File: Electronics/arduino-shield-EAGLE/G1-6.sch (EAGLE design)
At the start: 23 parts

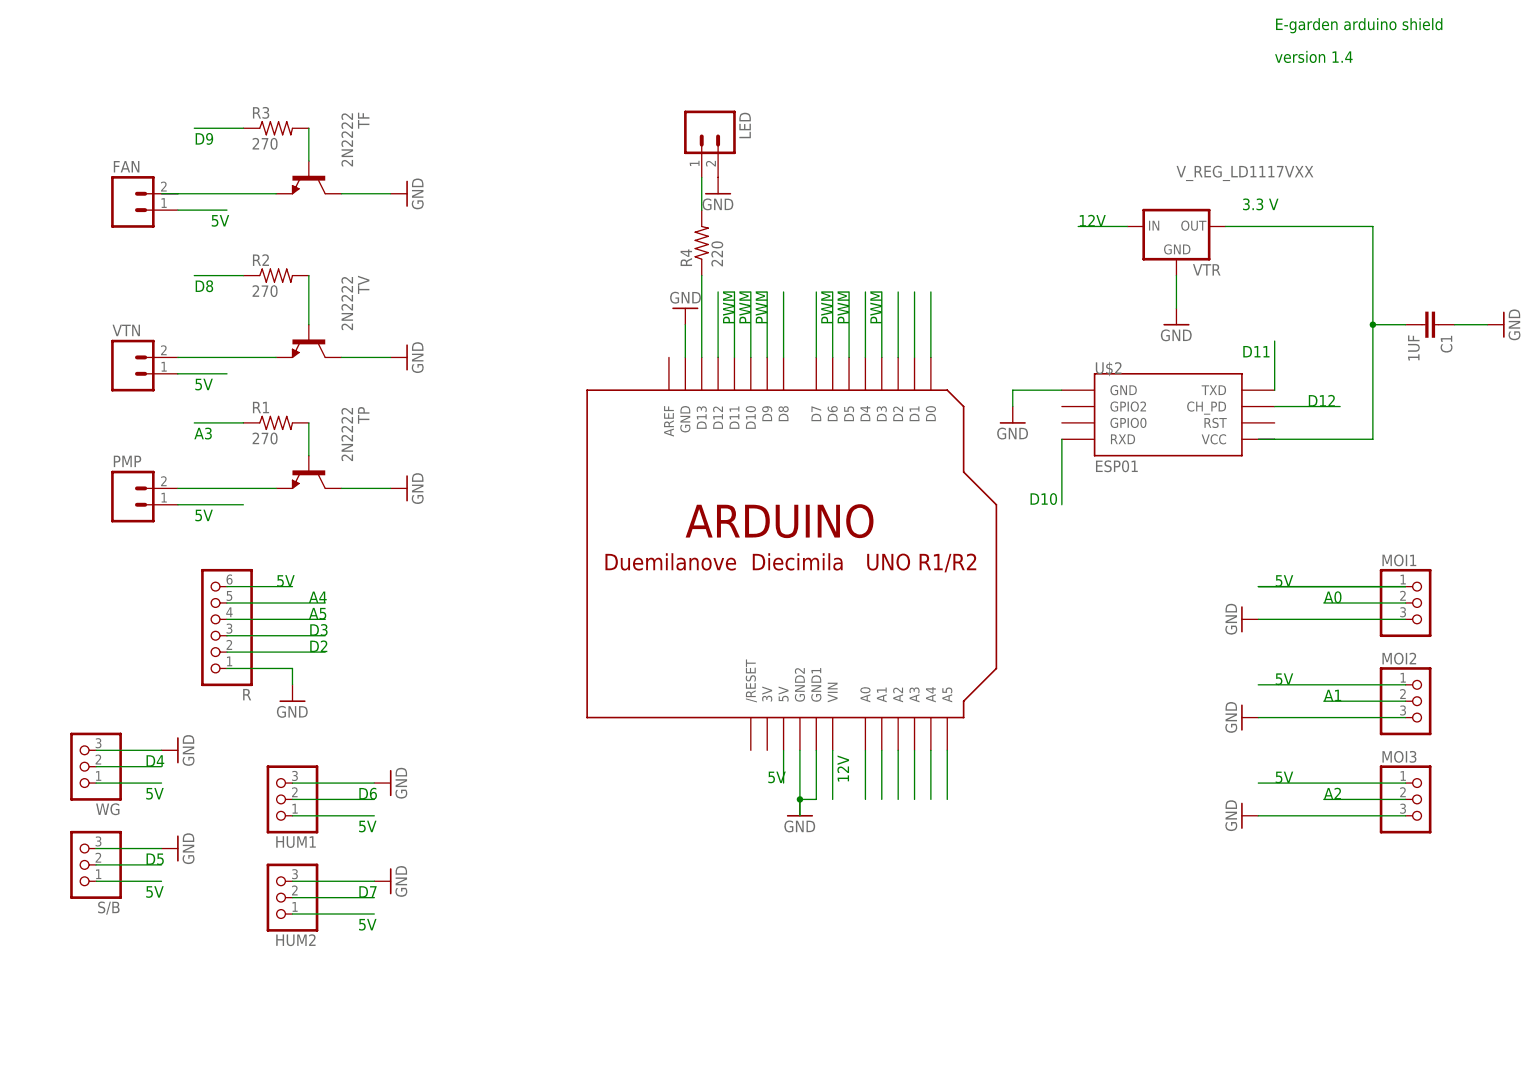
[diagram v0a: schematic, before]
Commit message: shield version 1.6
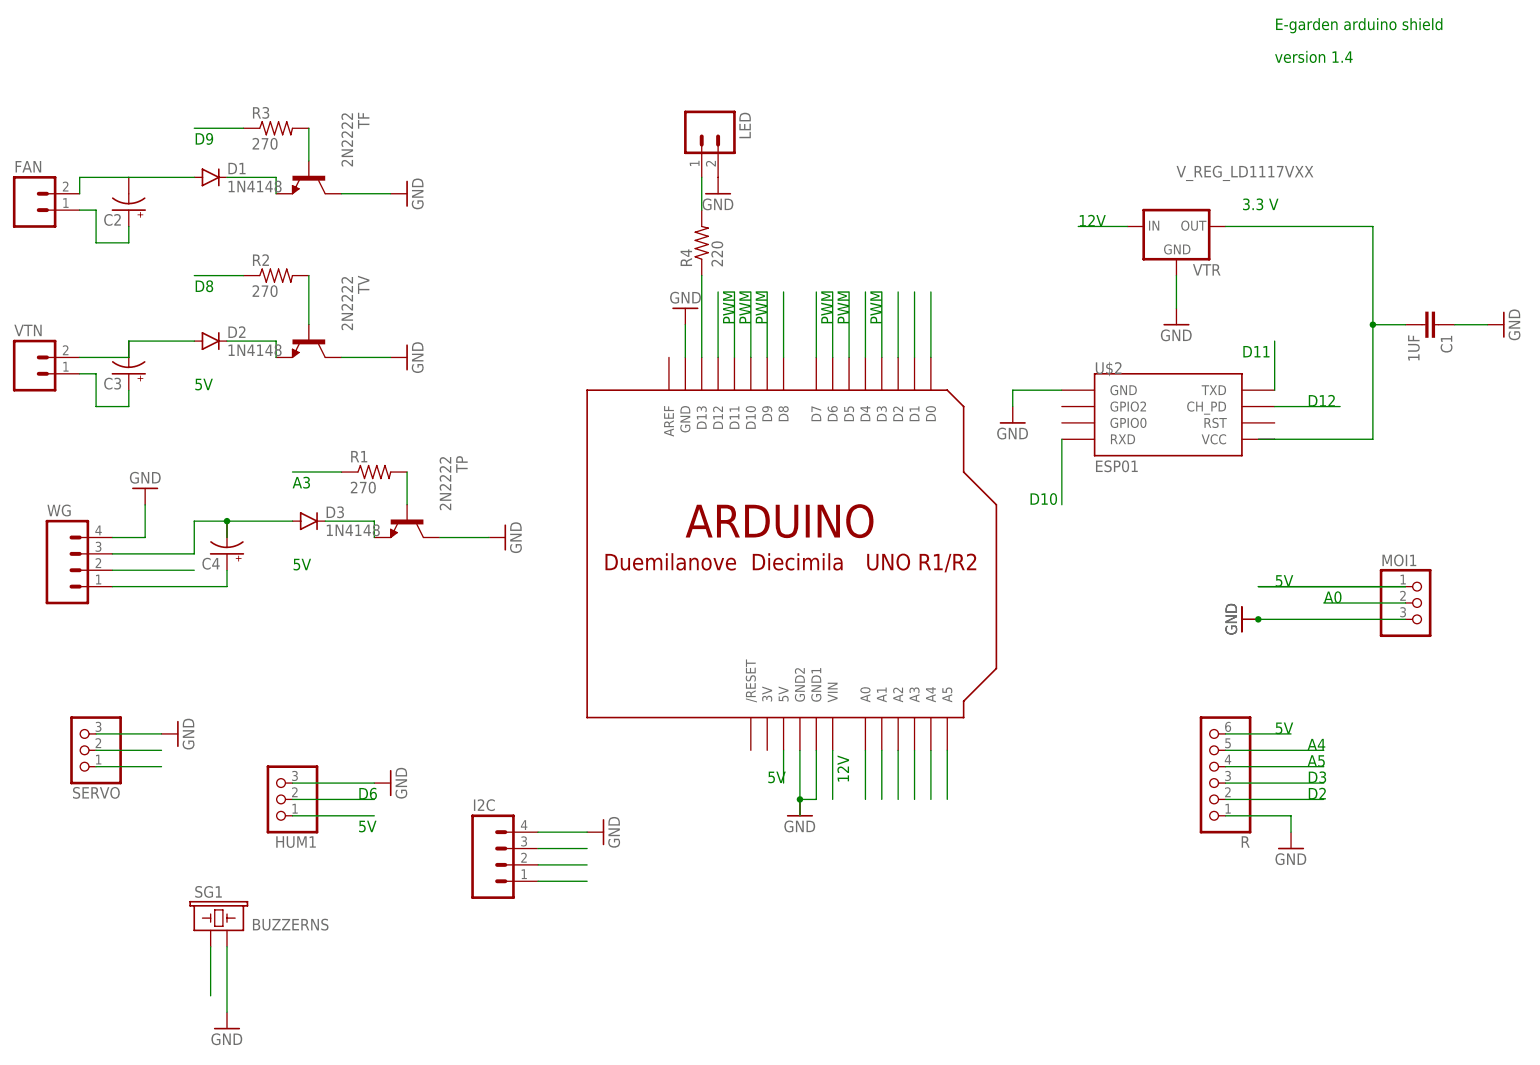
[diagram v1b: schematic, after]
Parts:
- removed HUM2, MOI2, MOI3, S/B: (no value), adafruit:PINHD-1X3CB
- removed PMP: (no value), SparkFun-Connectors:M02PTH
- added C2, C3, C4: (no value), SparkFun-Passives:CAP_POLPTH2
- added D1, D2, D3: 1N4148, SparkFun-DiscreteSemi:DIODE1N4148
- added I2C: (no value), SparkFun-Connectors:M04NO_SILK_ALL_ROUND
- added SERVO: (no value), adafruit:PINHD-1X3CB
- added SG1: BUZZERNS, SparkFun-Electromechanical:BUZZERNS
- WG: device adafruit:PINHD-1X3CB -> SparkFun-Connectors:M04NO_SILK_ALL_ROUND
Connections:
- removed net VTR: TV.E, VTN.2
- new net N$10: C4.-, D3.A, WG.3
- new net N$3: D2.C, TV.E
- new net N$6: C3.-, D2.A, VTN.2
- new net N$9: C2.-, D1.A, FAN.2
- net A1: now also WG.2; no longer MOI2.2
- net A2: now also R.4; no longer MOI3.2
- net A3: now also R.5; no longer R1.1
- net A4: now also I2C.3; no longer R.5
- net A5: now also I2C.2; no longer R.4
- net D2: now also R.3; no longer R.2
- net D3: now also R.2; no longer R.3
- net D4: now also SERVO.2; no longer WG.2
- net D5: now also SG1.1; no longer S/B.2
- net D7: now also R1.1; no longer HUM2.2
- net GND: now also I2C.4, SERVO.3, SG1.2, WG.4; no longer HUM2.3, MOI2.3, MOI3.3, S/B.3, WG.3
- net N$1: now also D1.C; no longer FAN.2
- net N$4: now also D3.C; no longer PMP.2
- net V5: now also C2.+, C3.+, C4.+, I2C.1, SERVO.1; no longer HUM2.1, MOI2.1, MOI3.1, PMP.1, S/B.1
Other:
- note removed: "A1"
- note removed: "A2"
- note removed: "D4"
- note removed: "D5"
- note removed: "D7"
- moved on the sheet: FAN, R, R1, TP, VTN
